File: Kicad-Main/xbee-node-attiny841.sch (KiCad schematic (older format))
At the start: 41 parts, among them P10 CONN_1, P11 CONN_1, P12 CONN_1, P13 CONN_1, P14 CONN_1, P15 CONN_1, P16 CONN_1, P17 CONN_1, P18 CONN_1, P19 CONN_1, P2 XBee Adaptor, P20 CONN_1, P3 Debug Adaptor, P7 CONN_1, P8 CONN_1, P9 CONN_1, Q1 BSS84, Q2 MMBT3904, Q3 2N7002, U1 ATTINY841, U2 MAX952ESA, U3 TPS77033

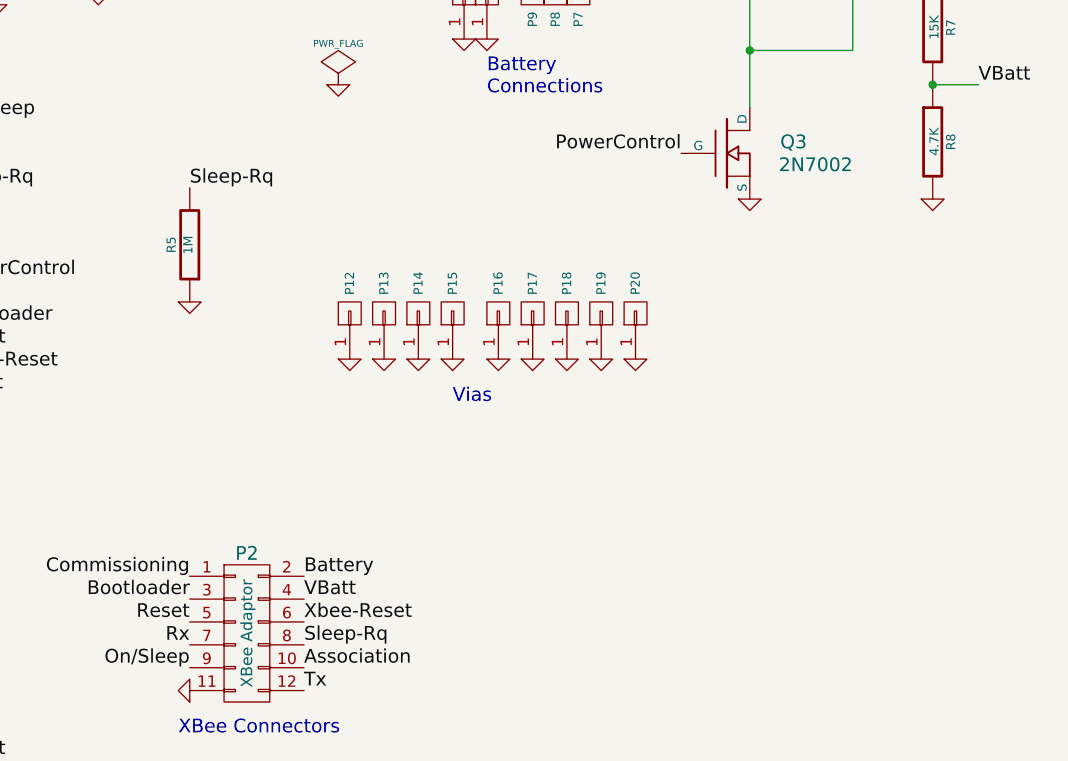
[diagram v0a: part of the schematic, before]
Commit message: Minor tweaks on the PCBs ready to manufacture
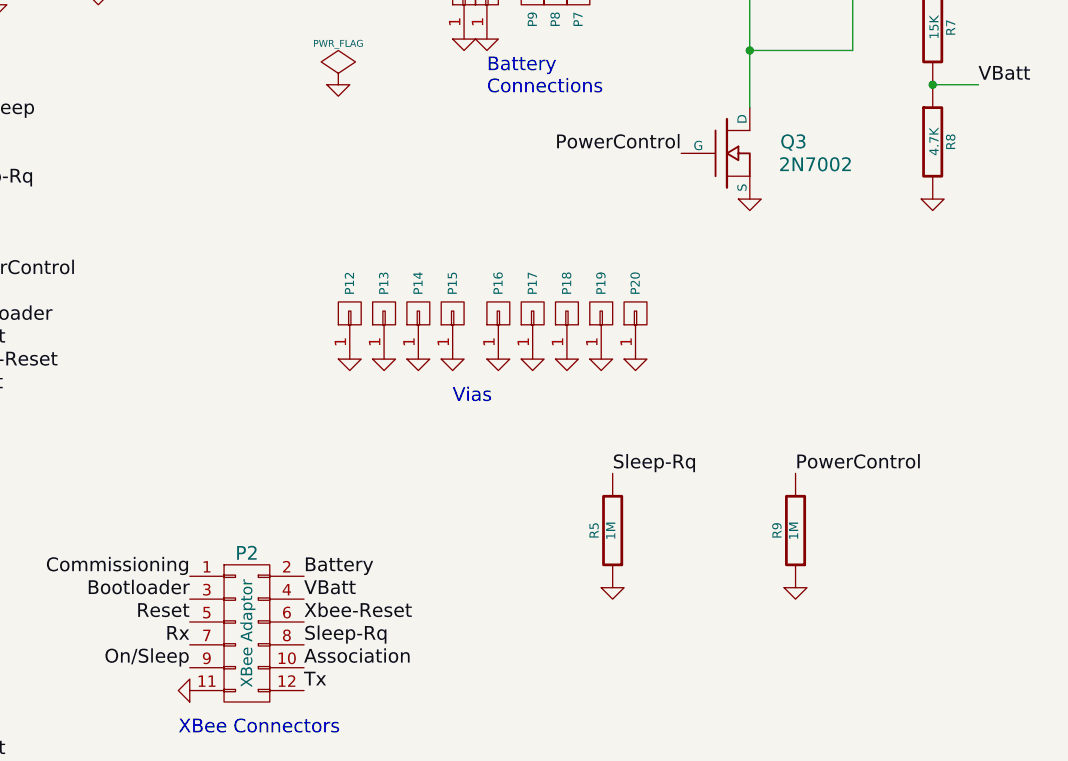
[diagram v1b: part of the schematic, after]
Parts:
- added R9: 1M, PhotoDiode:SM0603_Resistor, symbol R-RESCUE-xbee-node-attiny841
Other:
- moved on the sheet: R5
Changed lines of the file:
@@
 LIBS:TransistorParts
 LIBS:Sensors
+LIBS:xbee-node-attiny841-cache
 EELAYER 25 0
 EELAYER END
@@
 L R-RESCUE-xbee-node-attiny841 R5
 U 1 1 54823620
-P 7000 3000
-F 0 "R5" V 7080 3000 40  0000 C CNN
-F 1 "1M" V 7007 3001 40  0000 C CNN
-F 2 "PhotoDiode:SM0603_Resistor" V 6930 3000 30  0001 C CNN
-F 3 "" H 7000 3000 30  0000 C CNN
-	1    7000 3000
+P 8850 4250
+F 0 "R5" V 8930 4250 40  0000 C CNN
+F 1 "1M" V 8857 4251 40  0000 C CNN
+F 2 "PhotoDiode:SM0603_Resistor" V 8780 4250 30  0001 C CNN
+F 3 "" H 8850 4250 30  0000 C CNN
+	1    8850 4250
 	-1   0    0    1
 $EndComp
@@
 L GND-RESCUE-xbee-node-attiny841 #PWR034
 U 1 1 5482395B
-P 7000 3250
-F 0 "#PWR034" H 7000 3250 30  0001 C CNN
-F 1 "GND" H 7000 3180 30  0001 C CNN
-F 2 "" H 7000 3250 60  0000 C CNN
-F 3 "" H 7000 3250 60  0000 C CNN
-	1    7000 3250
-	1    0    0    -1
-$EndComp
-Text Label 7000 2750 0    60   ~ 0
+P 8850 4500
+F 0 "#PWR034" H 8850 4500 30  0001 C CNN
+F 1 "GND" H 8850 4430 30  0001 C CNN
+F 2 "" H 8850 4500 60  0000 C CNN
+F 3 "" H 8850 4500 60  0000 C CNN
+	1    8850 4500
+	1    0    0    -1
+$EndComp
+Text Label 8850 4000 0    60   ~ 0
 Sleep-Rq
 $Comp
@@
 	0    -1   -1   0
 $EndComp
+$Comp
+L R-RESCUE-xbee-node-attiny841 R9
+U 1 1 589265FC
+P 9650 4250
+F 0 "R9" V 9730 4250 40  0000 C CNN
+F 1 "1M" V 9657 4251 40  0000 C CNN
+F 2 "PhotoDiode:SM0603_Resistor" V 9580 4250 30  0001 C CNN
+F 3 "" H 9650 4250 30  0000 C CNN
+	1    9650 4250
+	-1   0    0    1
+$EndComp
+$Comp
+L GND-RESCUE-xbee-node-attiny841 #PWR?
+U 1 1 589266AB
+P 9650 4500
+F 0 "#PWR?" H 9650 4500 30  0001 C CNN
+F 1 "GND" H 9650 4430 30  0001 C CNN
+F 2 "" H 9650 4500 60  0000 C CNN
+F 3 "" H 9650 4500 60  0000 C CNN
+	1    9650 4500
+	1    0    0    -1
+$EndComp
+Text Label 9650 4000 0    60   ~ 0
+PowerControl
 $EndSCHEMATC
